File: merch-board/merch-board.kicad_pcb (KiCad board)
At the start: 2 copper layers, 86 x 54 mm, 84 parts, among them J1 Piano pads, P1 USB_C_Plug, SW1 BOOTSEL, SW2 RESET, SW3 OCT_DOWN, SW4 OCT_UP, SW5 TONE_SEL, U1 NCP1117-3.3_SOT223, U2 W25Q128JVS, U3 RP2040, U4 PCM5100A, U5 TPA6211A1DGN, U6 CY8CMBR3116, Y1 ABM8-272-T3

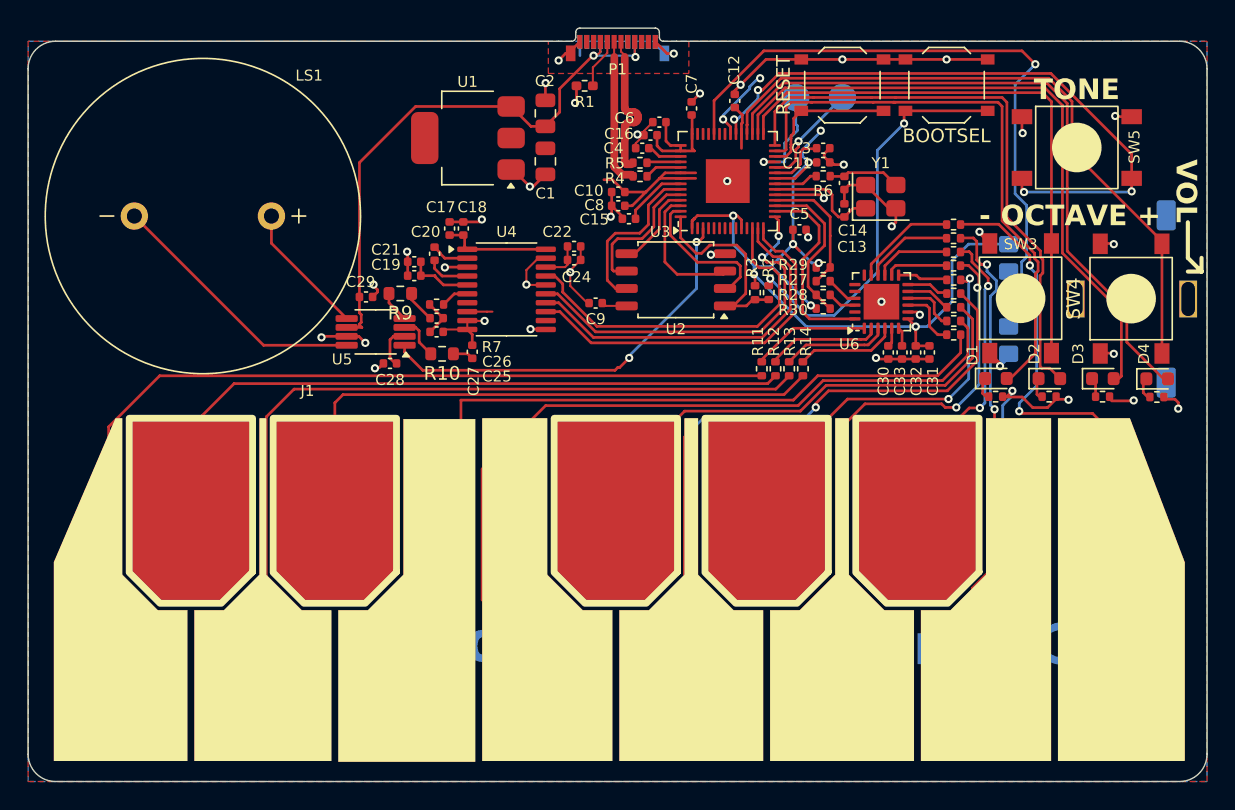
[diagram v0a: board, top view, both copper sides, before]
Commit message: Add artwork
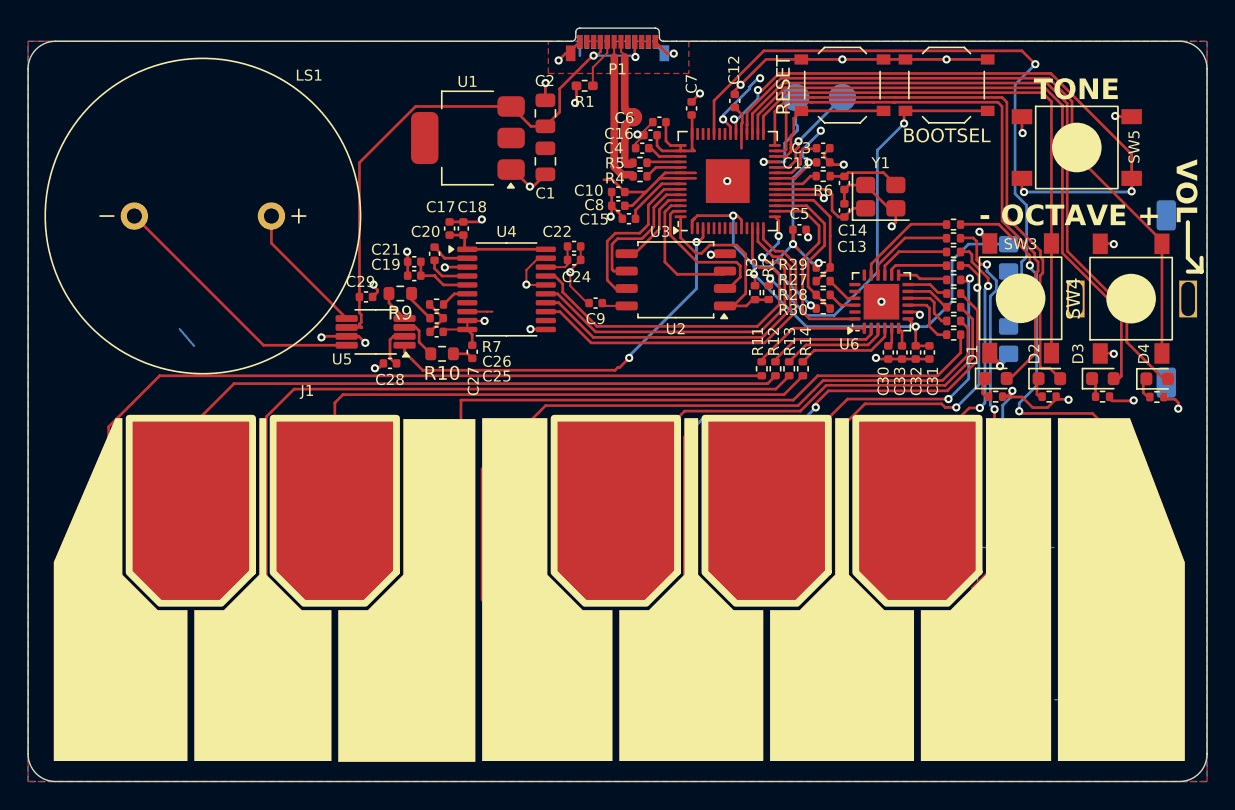
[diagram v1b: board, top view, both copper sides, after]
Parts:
- added REF**: LOGO, artsfest-art:Logo-ArtsCluster, B.Cu at (169.1, 112.5)
- added REF**: Building, artsfest-art:Building, B.Cu at (127.3, 105.7)
- added REF**: Logo-Artsfest, artsfest-art:Logo-Artsfest, B.Cu at (181.8, 112.7)
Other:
- board text added: "Design @kaine119"
- board text removed: "Cu cutout"
- board text removed: "Exposed Cu"
- board text removed: "Silkscreen"
